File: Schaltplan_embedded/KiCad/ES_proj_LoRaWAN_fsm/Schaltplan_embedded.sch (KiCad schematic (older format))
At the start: 0 parts

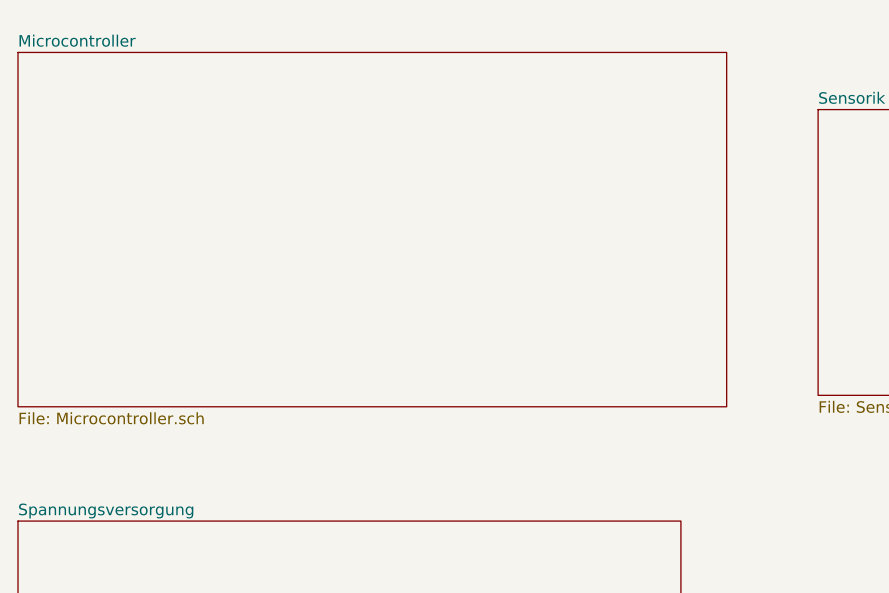
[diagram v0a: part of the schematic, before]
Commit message: Neuer Schaltplan
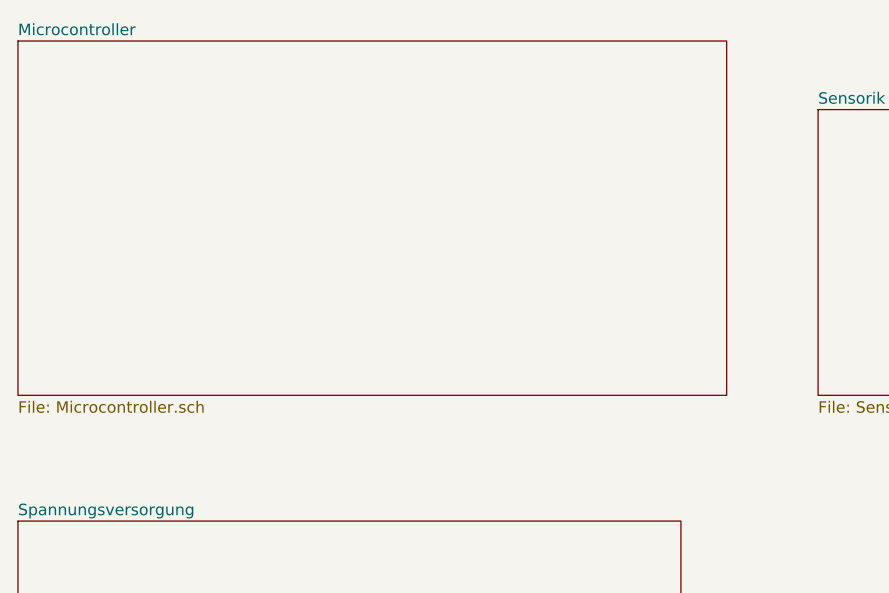
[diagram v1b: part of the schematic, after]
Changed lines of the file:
@@
 $EndDescr
 $Sheet
-S 950  850  3100 1550
+S 950  800  3100 1550
 U 5DC1A511
 F0 "Microcontroller" 50
